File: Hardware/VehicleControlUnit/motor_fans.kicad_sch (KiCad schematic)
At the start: 13 parts, among them IC3 EMC2305-1-AP-TR, J13 Fan_Debug_Conn

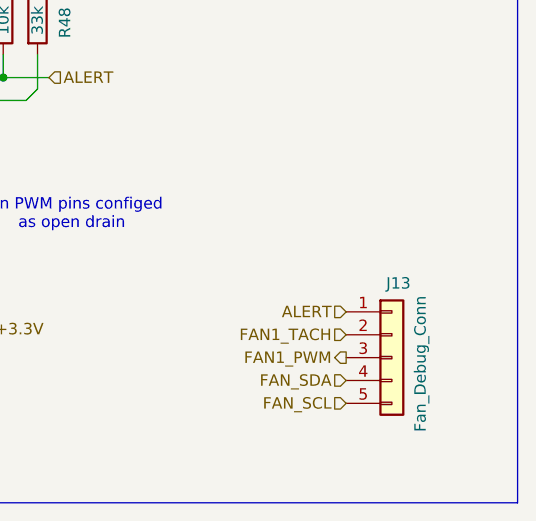
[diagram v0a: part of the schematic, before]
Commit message: VCU hardware prod files done night night
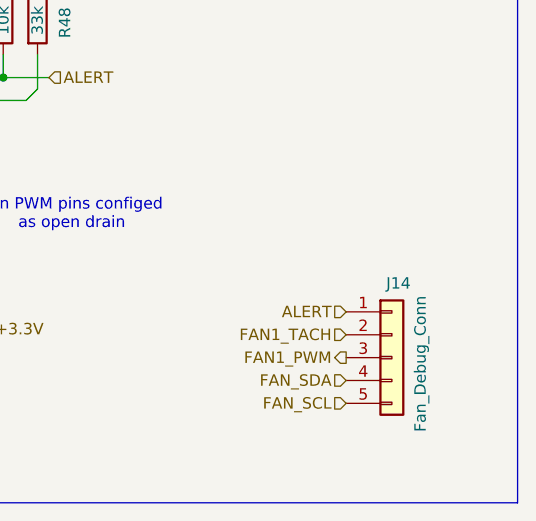
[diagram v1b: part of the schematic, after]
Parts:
- renumbered J13 to J14
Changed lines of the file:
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@@
 		(in_pos_files yes)
 		(dnp no)
-		(property "Reference" "J13"
+		(property "Reference" "J14"
 			(at 155.575 72.39 0)
 			(show_name no)
@@
 			(project "VehicleControlUnit"
 				(path "/e864fac9-3897-46c9-9101-6d5488c6cd3a/76867641-26a4-43d1-a64a-9a6eb791f3f7"
-					(reference "J13")
+					(reference "J14")
 					(unit 1)
 				)

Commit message: surabhi review pls
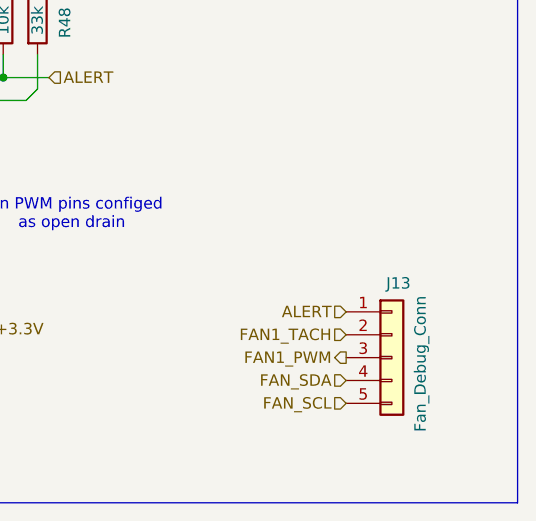
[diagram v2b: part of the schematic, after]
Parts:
- renumbered J14 to J13
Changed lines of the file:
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@@
 		(in_pos_files yes)
 		(dnp no)
-		(property "Reference" "J14"
+		(property "Reference" "J13"
 			(at 155.575 72.39 0)
 			(show_name no)
@@
 			(project "VehicleControlUnit"
 				(path "/e864fac9-3897-46c9-9101-6d5488c6cd3a/76867641-26a4-43d1-a64a-9a6eb791f3f7"
-					(reference "J14")
+					(reference "J13")
 					(unit 1)
 				)
